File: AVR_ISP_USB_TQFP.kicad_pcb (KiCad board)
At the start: 2 copper layers, 47 x 20 mm, 26 parts, among them CON1 USB-MICRO-B, IC1 ATMEGA8-AI, P1 CONN_02X05, P2 CONN_01X01, P3 CONN_01X01, P4 CONN_01X01, P5 CONN_01X01, X1 12MHz

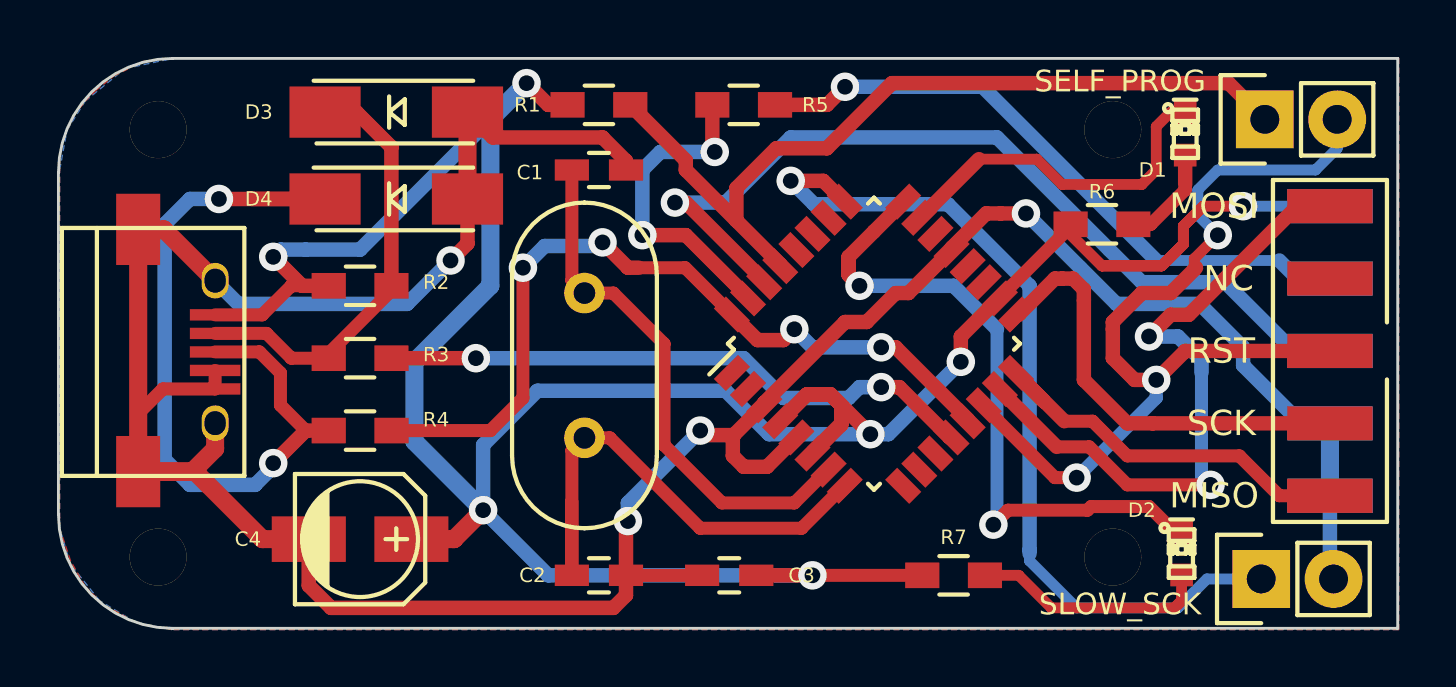
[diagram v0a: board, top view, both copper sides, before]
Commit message: final_v1
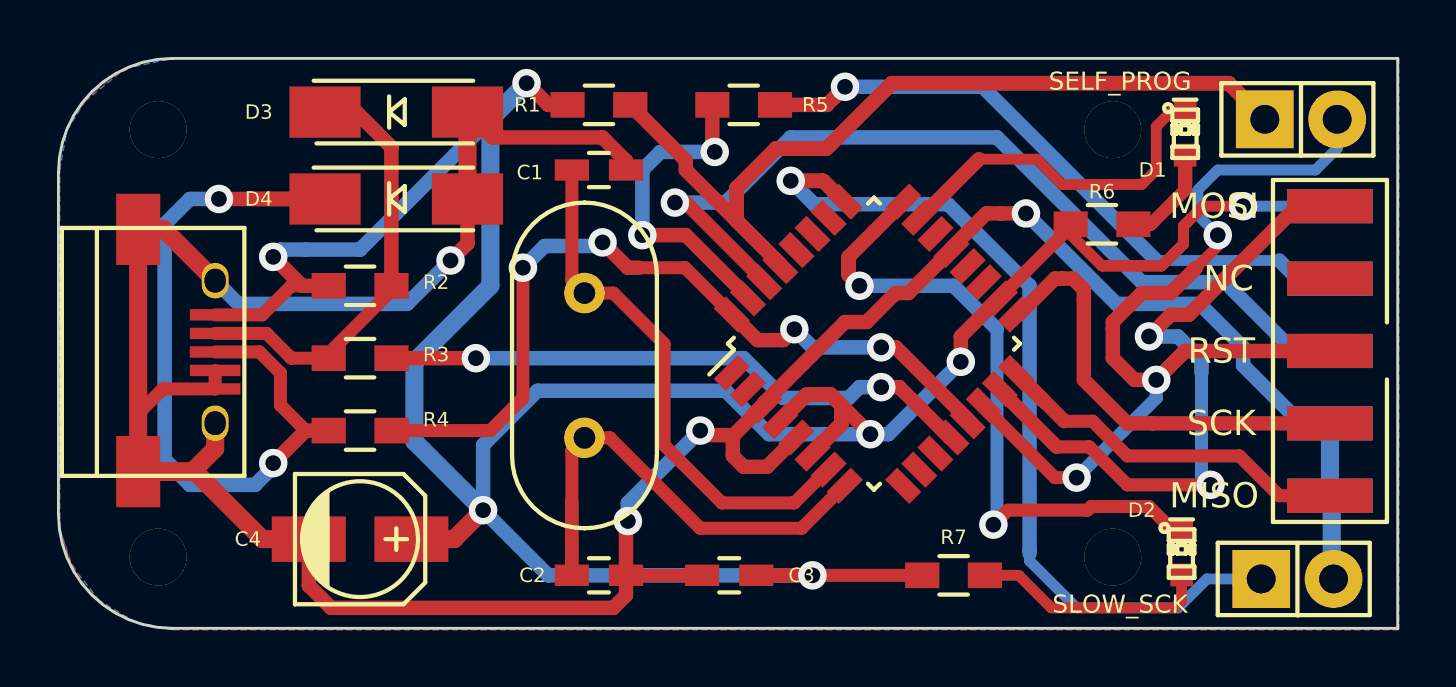
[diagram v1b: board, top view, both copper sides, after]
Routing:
- net Net-(IC1-Pad29): track 29.6 -> 53.5 mm
- net GND: track 110.6 -> 113.6 mm
- net Net-(IC1-Pad25): track 31.8 -> 34.0 mm
- net Net-(IC1-Pad14): track 32.3 -> 33.8 mm
